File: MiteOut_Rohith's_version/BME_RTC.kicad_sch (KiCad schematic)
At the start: 11 parts, among them J5 Conn_01x04_Socket, J6 Conn_01x04_Socket, J7 Conn_01x04_Socket, J8 Conn_01x04_Socket, SW5 SW_Push, U15 DS3231M

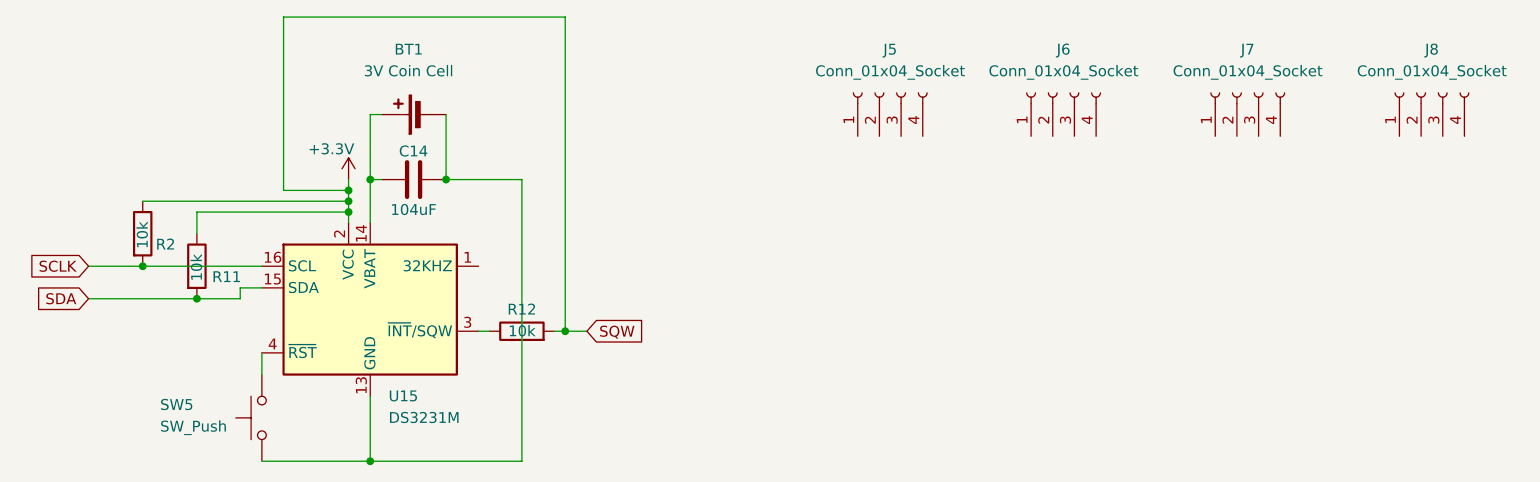
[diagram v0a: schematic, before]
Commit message: some changes ig
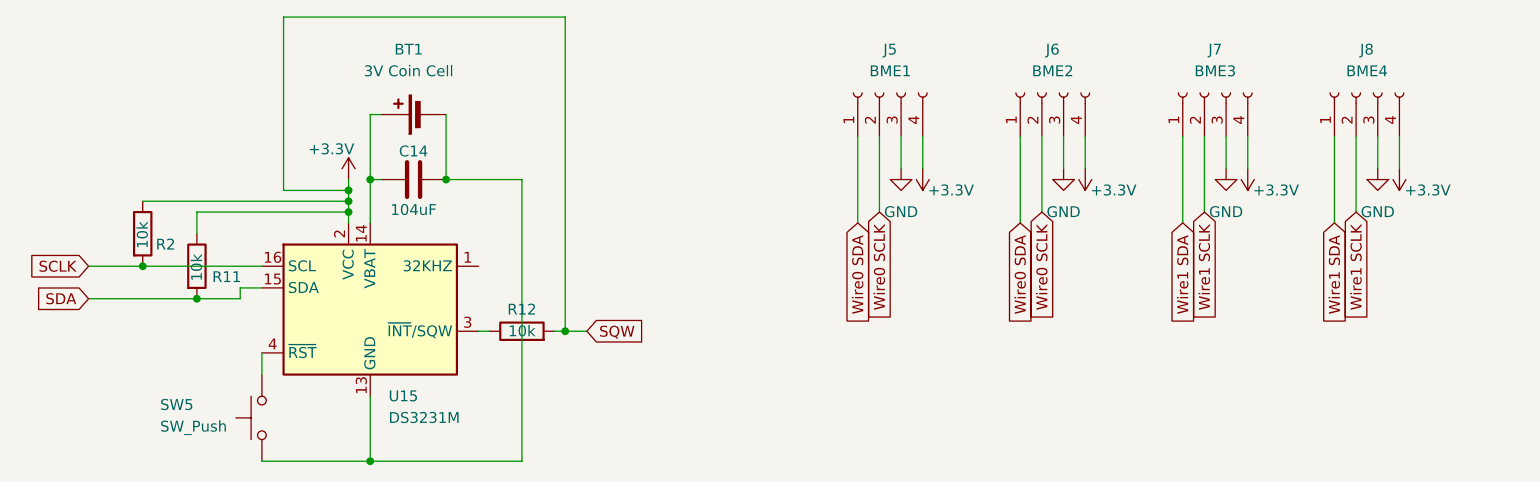
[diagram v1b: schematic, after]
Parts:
- J5: value Conn_01x04_Socket -> BME1
- J6: value Conn_01x04_Socket -> BME2
- J7: value Conn_01x04_Socket -> BME3
- J8: value Conn_01x04_Socket -> BME4
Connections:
- net +3.3V: now also J5.4 (Pin_4), J6.4 (Pin_4), J7.4 (Pin_4), J8.4 (Pin_4)
- net Wire0 SDA: now reaches J6.1 (Pin_1)
- net Wire0 SDA: now also J5.1 (Pin_1)
- net Wire0 SCLK: now reaches J6.2 (Pin_2)
- net Wire0 SCLK: now also J5.2 (Pin_2)
- net GND: now reaches J6.3 (Pin_3)
- net GND: now also J5.3 (Pin_3), J7.3 (Pin_3), J8.3 (Pin_3)
- net Wire1 SDA: now reaches J7.1 (Pin_1)
- net Wire1 SDA: now also J8.1 (Pin_1)
- net Wire1 SCLK: now reaches J7.2 (Pin_2)
- net Wire1 SCLK: now also J8.2 (Pin_2)
